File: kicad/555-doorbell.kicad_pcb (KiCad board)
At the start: 2 copper layers, 44.7 x 41.7 mm, 14 parts, among them SW1 SW_PUSH_SMALL_H, U1 LM555N

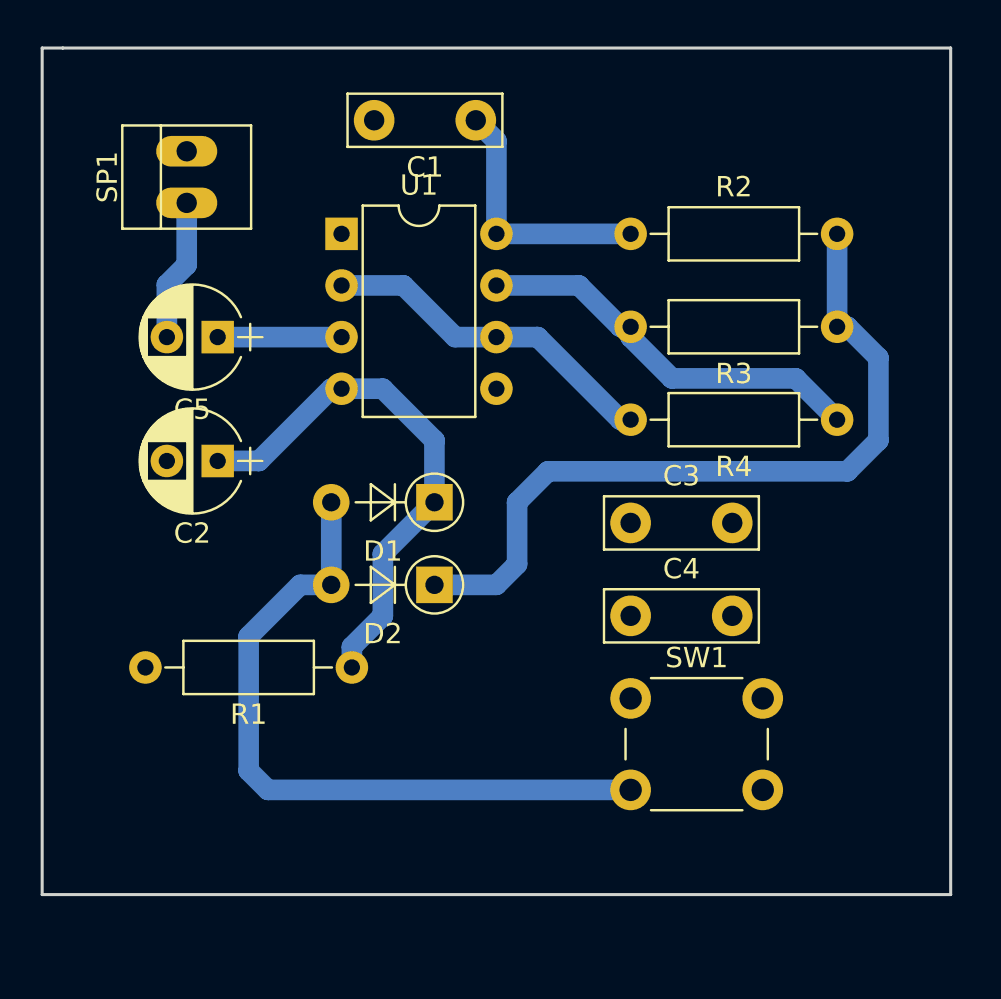
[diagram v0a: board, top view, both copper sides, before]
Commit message: pcb v1 finished
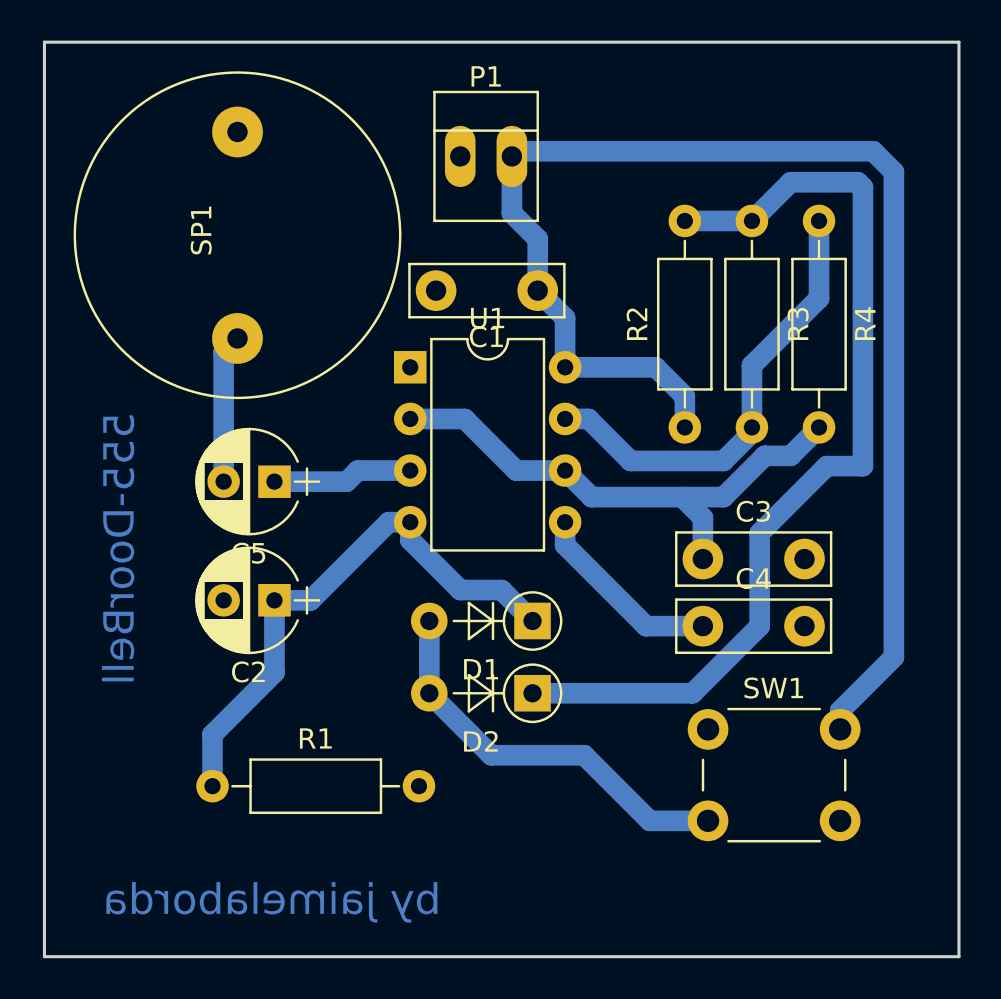
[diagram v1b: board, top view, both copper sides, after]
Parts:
- added P1: CONN_01X02, Connect:PINHEAD1-2, F.Cu at (140.5, 87.1)
- SP1: footprint Connect:PINHEAD1-2 -> Buzzers_Beepers:BUZZER
- moved R2 9.89 mm to (151.5, 100.5), turned to 90 degrees
- moved R4 9.82 mm to (158.1, 90.3), turned to 270 degrees
- moved R1 9.01 mm to (128.3, 118.1), turned to 0 degrees
- moved C1 8.92 mm to (144.3, 93.7)
- moved C5 7.64 mm to (131.3, 103.1)
- moved D1 7.58 mm to (144.0, 110.0)
- moved C2 7.41 mm to (131.3, 109.0)
- moved U1 7.39 mm to (138.0, 97.5)
- moved D2 7.19 mm to (144.0, 113.5)
- moved R3 6.68 mm to (154.8, 90.3), turned to 270 degrees
- moved SW1 4.10 mm to (152.7, 115.3)
- moved C3 3.98 mm to (152.4, 106.9)
- moved C4 3.59 mm to (152.4, 110.2)
- moved SP1 2.96 mm to (129.5, 91.0)
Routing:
- net VCC: track 12.6 -> 67.3 mm
- net Net-(D1-Pad2): track 35.0 -> 19.9 mm
- net Net-(C3-Pad1): track 17.0 -> 26.6 mm
- net Net-(C4-Pad1): track 0.00 -> 9.56 mm
- net Net-(D2-Pad1): track 37.9 -> 46.9 mm
- net Net-(R3-Pad2): track 19.8 -> 22.9 mm
- net Net-(C2-Pad1): track 26.1 -> 27.2 mm
- net Net-(C5-Pad1): track 6.10 -> 6.91 mm
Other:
- board size 44.7 x 41.7 mm -> 45 x 45 mm
- board text added: "555-DoorBell"
- board text added: "by jaimelaborda"
